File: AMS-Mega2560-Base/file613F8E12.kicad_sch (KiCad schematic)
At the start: 8 parts, among them IC18 MAX31865AAP+, J28 Conn_01x02, J29 Conn_01x03, J30 Conn_01x02

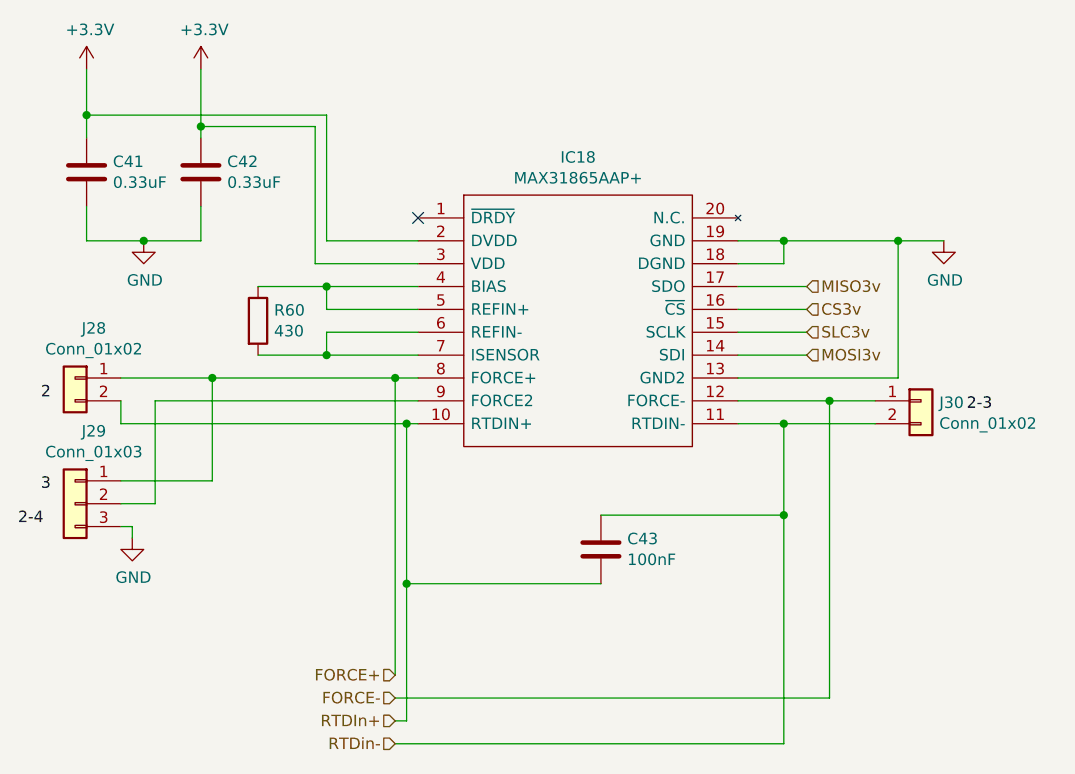
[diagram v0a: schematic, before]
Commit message: continuing pcb layout
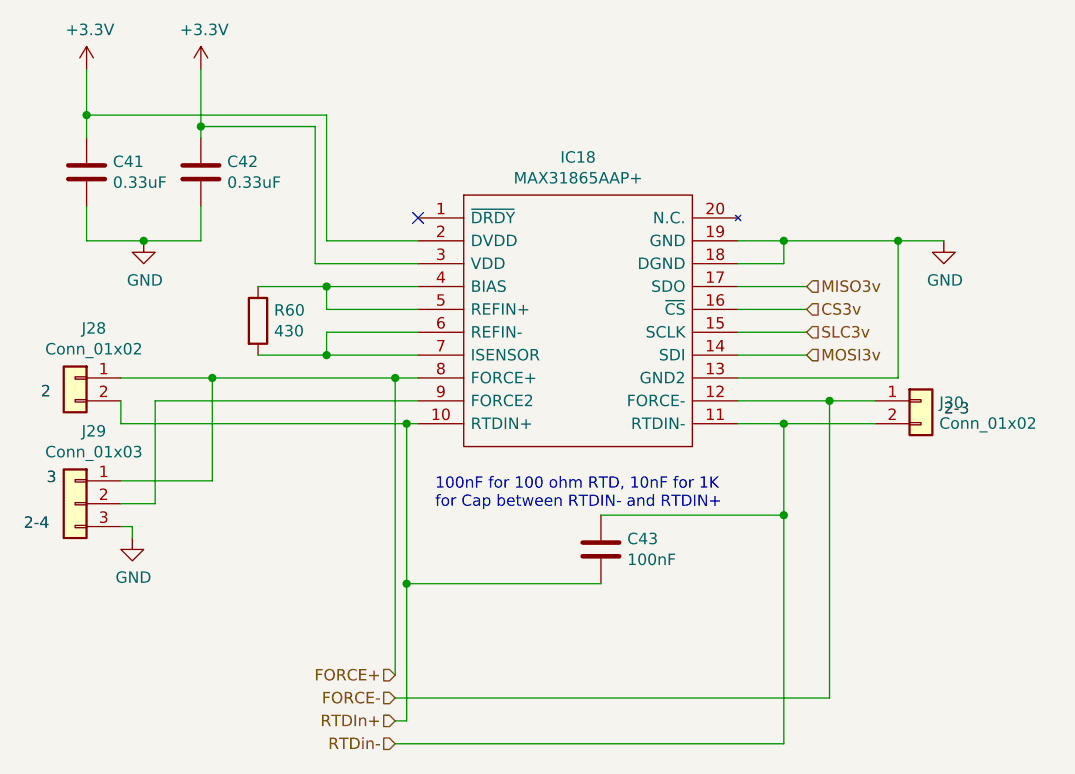
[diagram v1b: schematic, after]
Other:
- note added: "100nF for 100 ohm RTD, 10nF for 1K for Cap between RTDIN- and RTDIN+"
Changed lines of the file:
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@@
     (stroke (width 0) (type default) (color 0 0 0 0))
   )
-  (label "2-3" (at 196.85 99.06 0)
+  (text "100nF for 100 ohm RTD, 10nF for 1K\nfor Cap between RTDIN- and RTDIN+"
+    (at 137.795 109.855 0)
+    (effects (font (size 1.25 1.25)) (justify left bottom))
+  )
+  (label "2-3" (at 194.31 99.695 0)
     (effects (font (size 1.27 1.27)) (justify left bottom))
   )
@@
     (effects (font (size 1.27 1.27)) (justify left bottom))
   )
-  (label "2-4" (at 91.44 111.76 0)
+  (label "2-4" (at 92.075 112.395 0)
     (effects (font (size 1.27 1.27)) (justify left bottom))
   )
-  (label "3" (at 93.98 107.95 0)
+  (label "3" (at 94.615 107.315 0)
     (effects (font (size 1.27 1.27)) (justify left bottom))
   )
